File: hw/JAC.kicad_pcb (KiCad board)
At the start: 2 copper layers, 65.6 x 32.6 mm, 23 parts, among them J1 USB_C_Receptacle_USB2.0, Q1 AO3401A, SW1 BT0, U1 EPDM, U2 4056M, U3 RX-8025T, U4 ESP32-C3-WROOM-02

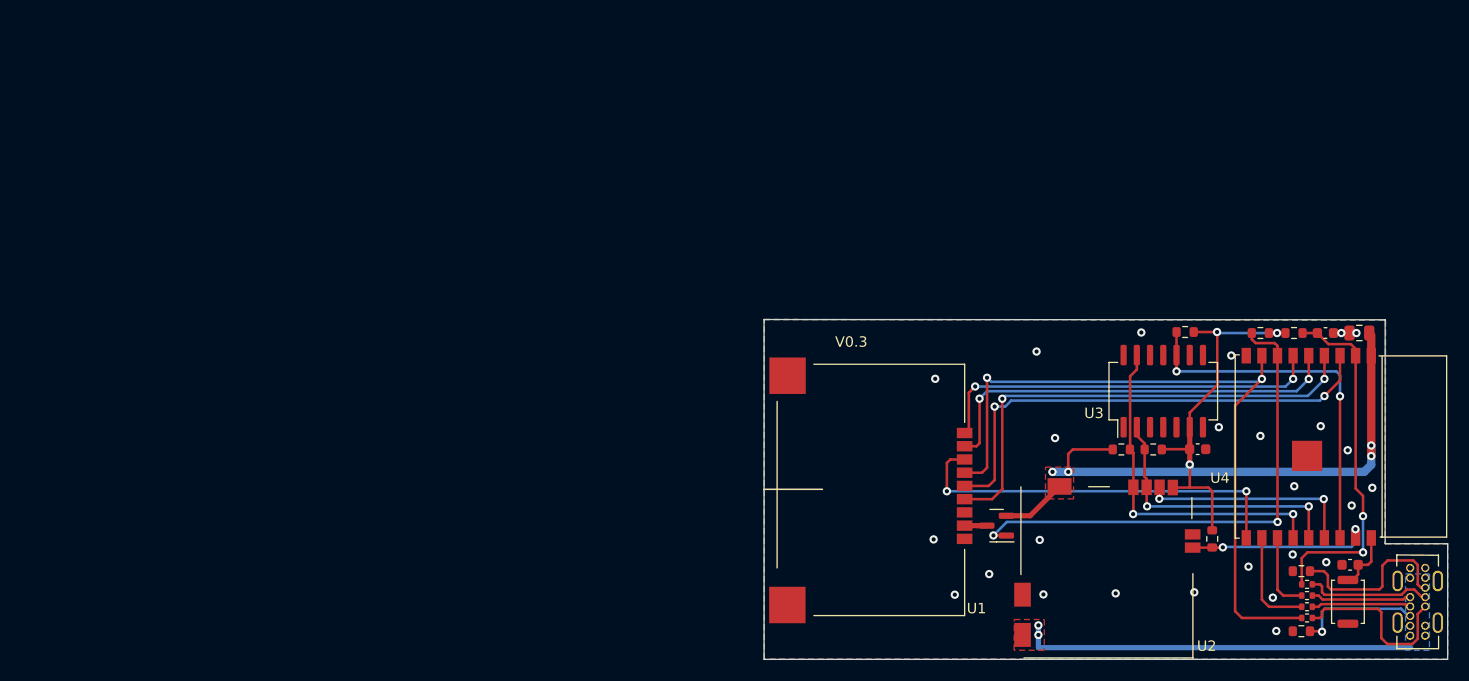
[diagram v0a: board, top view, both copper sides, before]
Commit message: hw: 4.2 inch screen variant
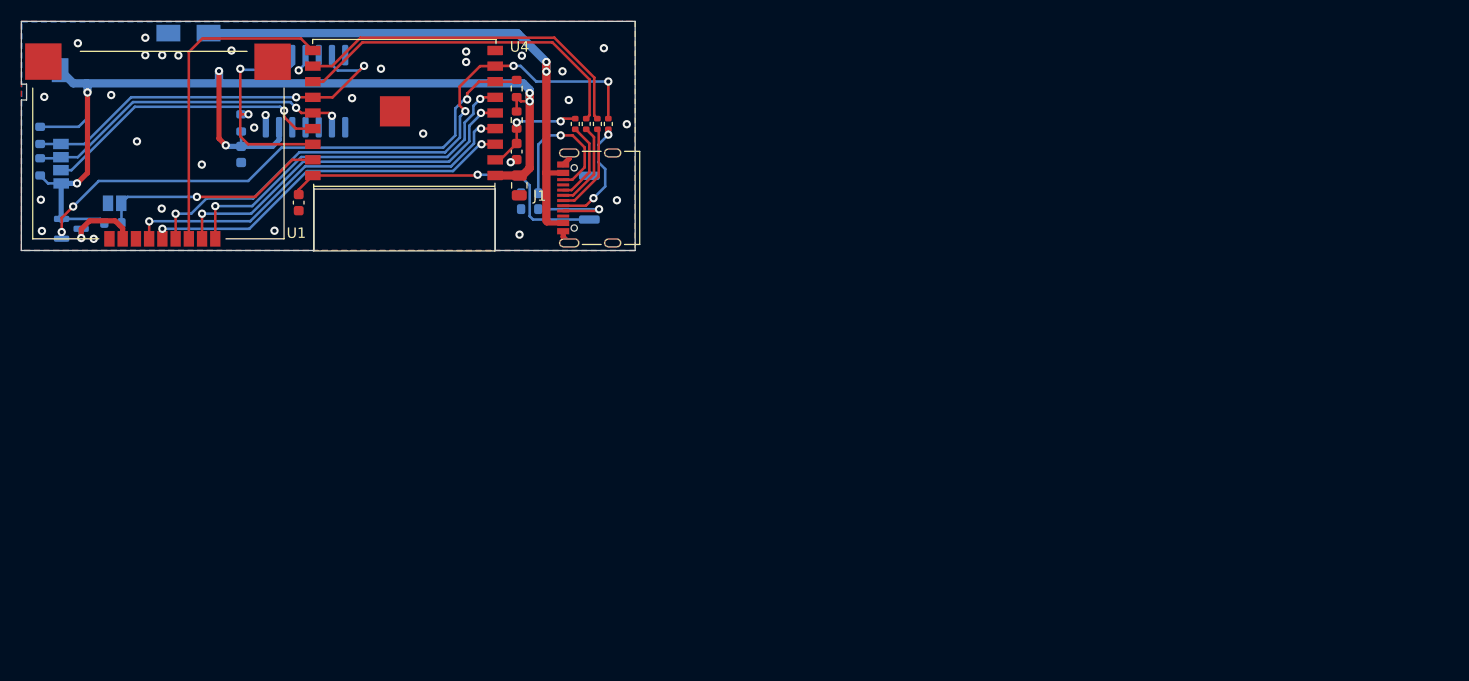
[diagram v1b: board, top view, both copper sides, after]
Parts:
- C3, Q1, R3, R4, R5, R6, R7, R8, SW1, U2, U3: moved to B.Cu
- J1: footprint Joke:TYPE-C-VERT -> Connector_USB:USB_C_Receptacle_Palconn_UTC16-G
- moved R7 110.2 mm to (78.0, 64.8), turned to 90 degrees
- moved R4 109.8 mm to (85.0, 70.2), turned to 0 degrees
- moved R8 108.1 mm to (78.0, 61.7), turned to -90 degrees
- moved C1 106.8 mm to (102.8, 68.2), turned to 90 degrees
- moved U2 100.3 mm to (86.6, 54.6), turned to -90 degrees
- moved C3 96.1 mm to (97.3, 63.6), turned to -90 degrees
- moved U4 95.2 mm to (112.9, 63.8), turned to 180 degrees
- moved Q1 93.3 mm to (81.0, 70.7), turned to 0 degrees
- moved R3 92.8 mm to (97.3, 60.5), turned to -90 degrees
- moved J1 88.5 mm to (130.7, 67.8)
- moved U3 87.2 mm to (103.5, 57.5)
- moved R5 84.4 mm to (125.0, 68.8)
- moved JP4 83.0 mm to (129.4, 60.6), turned to 90 degrees
- moved JP1 82.7 mm to (130.4, 60.6), turned to 90 degrees
- moved SW1 82.5 mm to (130.7, 67.7), turned to -90 degrees
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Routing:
- net /IO0: track 6.27 -> 32.5 mm, vias 0 -> 1
- net /TXD: track 7.53 -> 33.5 mm
- net /RXD: track 10.0 -> 33.8 mm
- net /CHIP_PU: track 34.2 -> 10.5 mm
- net VBUS: track 37.9 -> 53.1 mm
- net /IO2: track 35.3 -> 21.5 mm
- net /EPD_DC: track 69.9 -> 57.4 mm, vias 2 -> 4
- net +3V3: track 94.5 -> 106.5 mm, vias 7 -> 6
- net /EPD_RST: track 46.7 -> 36.3 mm
- net /EPD_BUSY: track 46.7 -> 39.2 mm
- net /ALRT: track 20.7 -> 27.9 mm, vias 2 -> 1
- net /FSPICS0: track 37.8 -> 30.9 mm, vias 2 -> 0
- net Net-(J1-PadB7): track 17.2 -> 10.9 mm, vias 0 -> 2
- net /I2C_SCL: track 25.7 -> 31.9 mm
- net /I2C_SDA: track 33.3 -> 38.6 mm
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- removed copper zone on F.Cu, net +3V3
- removed copper zone on B.Cu, net VBUS
- removed copper zone on F.Cu, net VBUS
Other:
- board size 65.6 x 32.6 mm -> 58.9 x 22 mm
- board text removed: "V0.3"
